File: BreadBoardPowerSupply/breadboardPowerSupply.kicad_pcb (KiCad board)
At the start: 2 copper layers, 17 parts, among them J1 Conn_01x02_Pin, J2 Conn_01x02_Pin, J3 Conn_01x03_Pin, J4 Conn_01x03_Pin, J5 Screw_Terminal_01x02, J6 Barrel_Jack_Switch, J7 Screw_Terminal_01x02, SW1 SW_Wuerth_450301014042, U1 LM7805_TO220, U2 LM317_TO-220

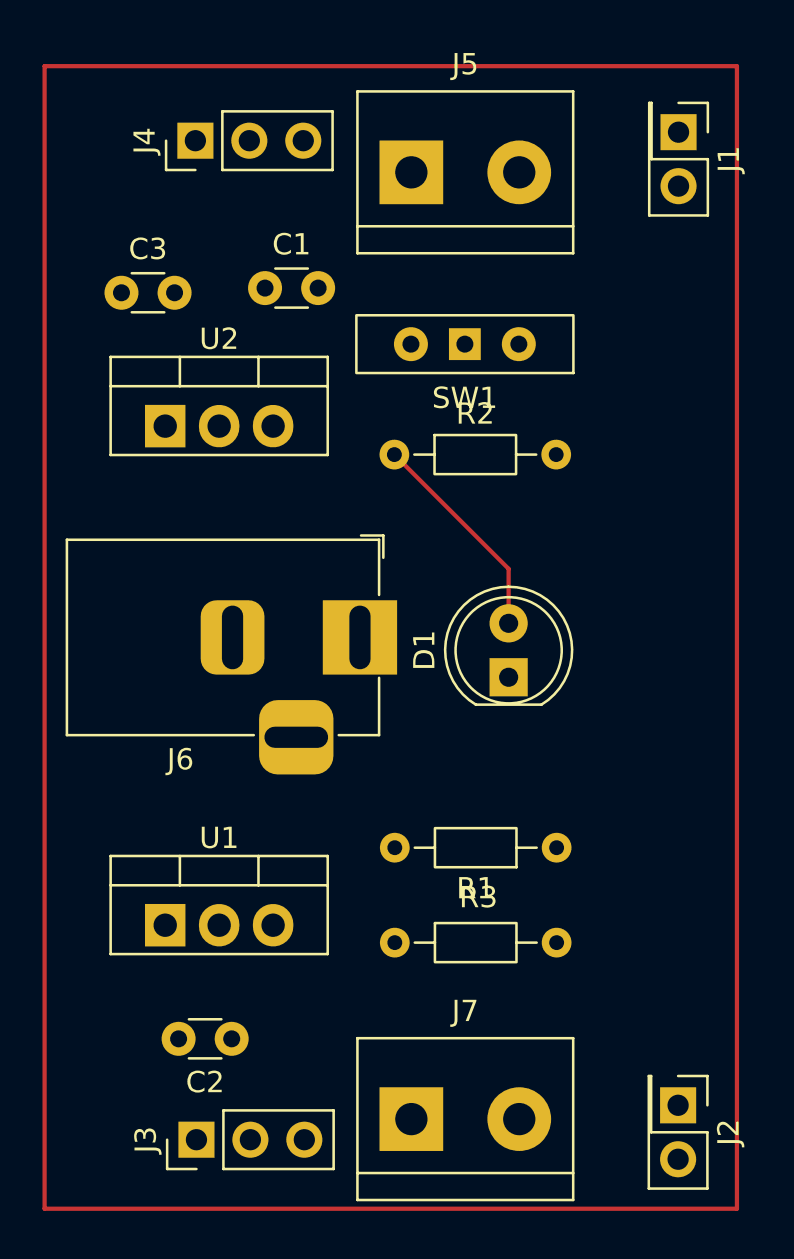
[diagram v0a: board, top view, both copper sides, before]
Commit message: Routed PCB
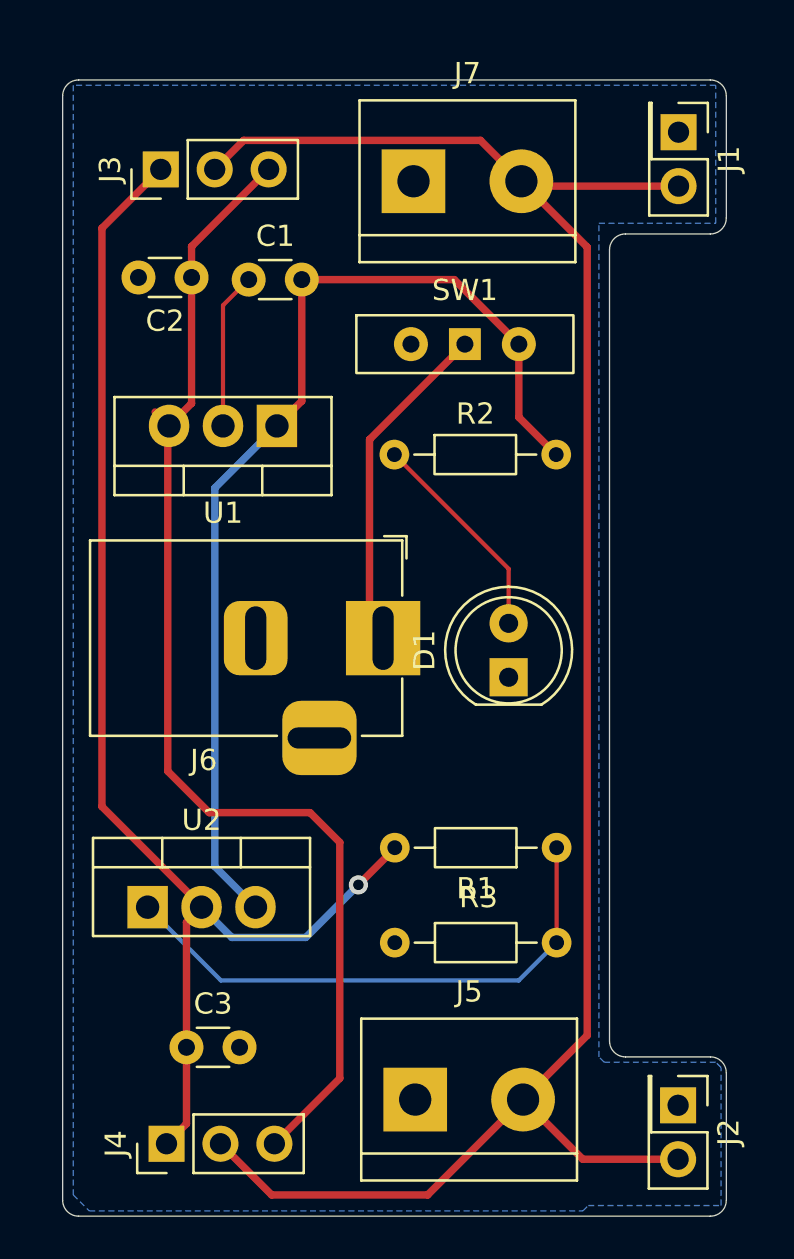
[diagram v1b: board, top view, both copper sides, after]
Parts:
- moved J4 47.2 mm to (145.9, 135.1)
- moved J3 45.7 mm to (145.6, 89.2)
- moved J7 44.2 mm to (157.5, 89.8)
- moved J5 43.7 mm to (157.6, 133.0)
- moved C2 35.9 mm to (147.1, 94.3)
- moved C3 35.7 mm to (146.8, 130.6)
- moved U1 24.1 mm to (151.1, 101.3), turned to 180 degrees
- moved U2 22.7 mm to (145.0, 124.0)
- moved J6 1.09 mm to (156.1, 111.3)
- moved C1 0.87 mm to (149.8, 94.4)
- turned SW1 to 0 degrees
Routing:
- net /PWR_output: track 0.00 -> 94.6 mm
- net /3.3V: track 0.00 -> 61.1 mm, vias 0 -> 1
- net /5V: track 0.00 -> 56.2 mm
- net /12V: track 0.00 -> 50.0 mm
- net Net-(U2-ADJ): track 0.00 -> 25.9 mm
- net /PWR_input: track 0.00 -> 16.0 mm
- net GND: track 0.00 -> 7.39 mm
- added copper zone on B.Cu, net GND
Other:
- board outline added: 31.2 x 53.5 mm
